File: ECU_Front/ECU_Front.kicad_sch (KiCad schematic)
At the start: 19 parts, among them J1 Conn_01x04_Pin, J3 Conn_01x02_Pin, U2 YAAJ_DCDC_StepDown_LM2596, U4 ESP32-DevKitC

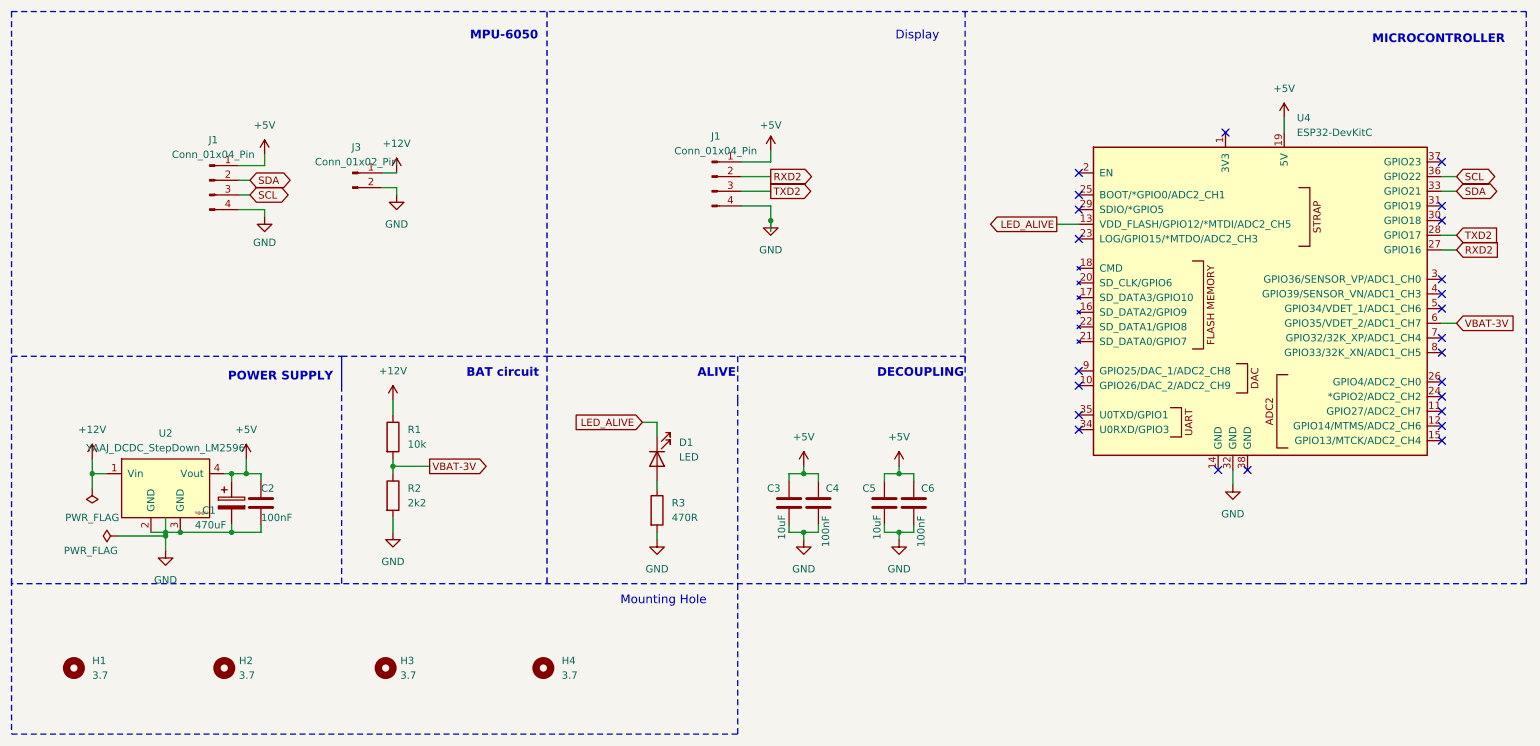
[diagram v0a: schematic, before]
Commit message: final fix ECU Front
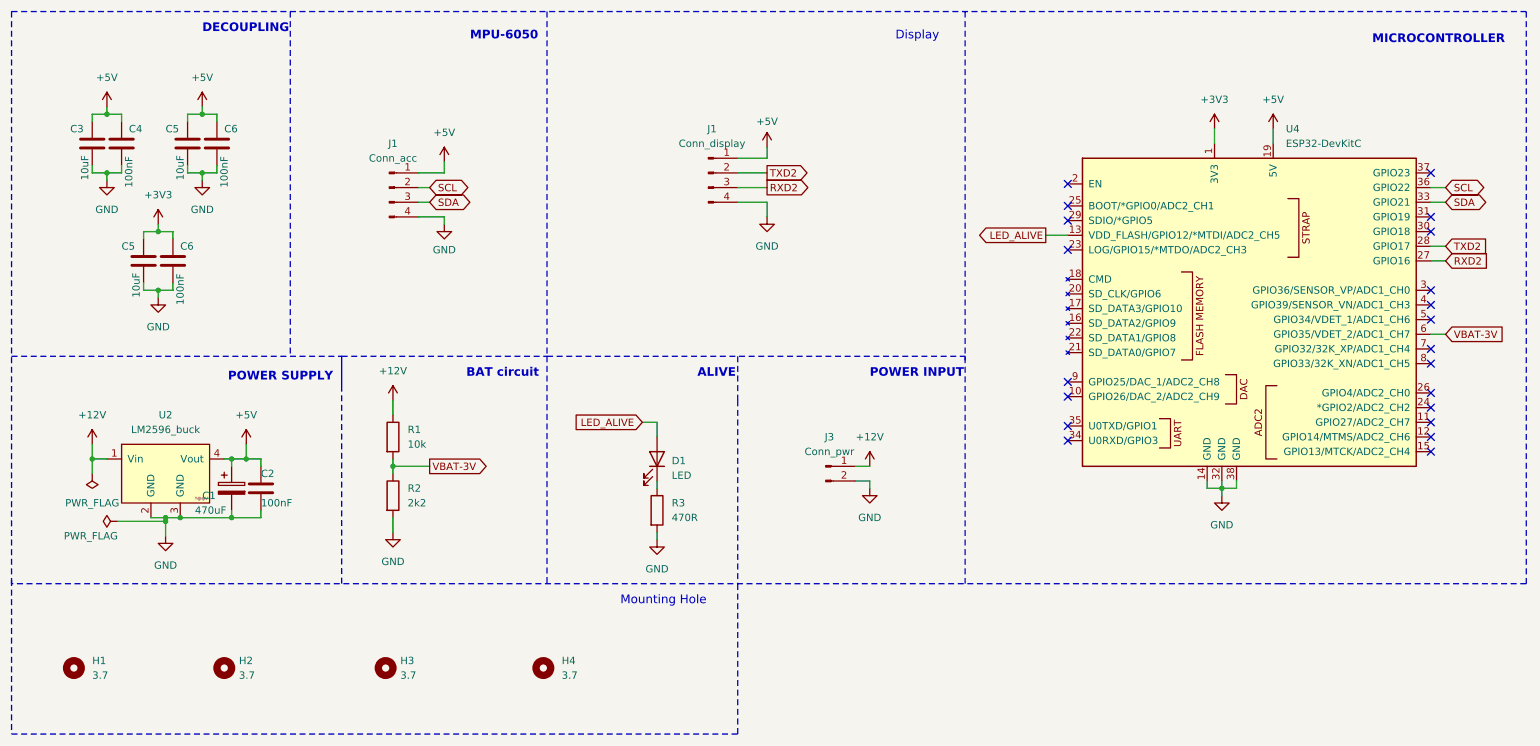
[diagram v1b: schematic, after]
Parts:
- added C5: 10uF, Capacitor_THT:C_Disc_D5.0mm_W2.5mm_P5.00mm, symbol Device:C
- added C6: 100nF, Capacitor_THT:C_Disc_D5.0mm_W2.5mm_P5.00mm, symbol Device:C
- D1: footprint LED_THT:LED_D3.0mm_FlatTop -> LED_THT:LED_D5.0mm
- J1: value Conn_01x04_Pin -> Conn_acc; footprint Connector:NS-Tech_Grove_1x04_P2mm_Vertical -> Connector_JST:JST_XH_B4B-XH-A_1x04_P2.50mm_Vertical
- J1: value Conn_01x04_Pin -> Conn_display; footprint Connector:NS-Tech_Grove_1x04_P2mm_Vertical -> Connector_JST:JST_XH_B4B-XH-A_1x04_P2.50mm_Vertical
- J3: value Conn_01x02_Pin -> Conn_pwr; footprint Connector_PinHeader_2.54mm:PinHeader_1x02_P2.54mm_Vertical -> Connector_JST:JST_XH_B2B-XH-A_1x02_P2.50mm_Vertical
- U2: value YAAJ_DCDC_StepDown_LM2596 -> LM2596_buck
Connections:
- net GND: now also U4.14 (GND), U4.38 (GND), C5.2, C6.2
- net LED_ALIVE: now also D1.2 (A); no longer D1.1 (K)
- net RXD2: now also J1.3 (Pin_3); no longer J1.2 (Pin_2)
- net SCL: now also J1.2 (Pin_2); no longer J1.3 (Pin_3)
- net SDA: now also J1.3 (Pin_3); no longer J1.2 (Pin_2)
- net TXD2: now also J1.2 (Pin_2); no longer J1.3 (Pin_3)
- net at R3.1: now also D1.1 (K); no longer D1.2 (A)
- net +3V3: now reaches U4.1 (3V3)
- net +3V3: now also C5.1, C6.1
- no-connect marks 24 -> 21
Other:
- note added: "POWER INPUT"
- moved on the sheet: C1, C2, C3, C4, C5, C6, D1, J1, J3, U2, U4
